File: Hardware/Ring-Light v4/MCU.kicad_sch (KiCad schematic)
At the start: 39 parts, among them U35 CC2640R2FRSMR, U38 W25X40CLUXIG_TR, Y1 32.768kHz, Y2 24MHz

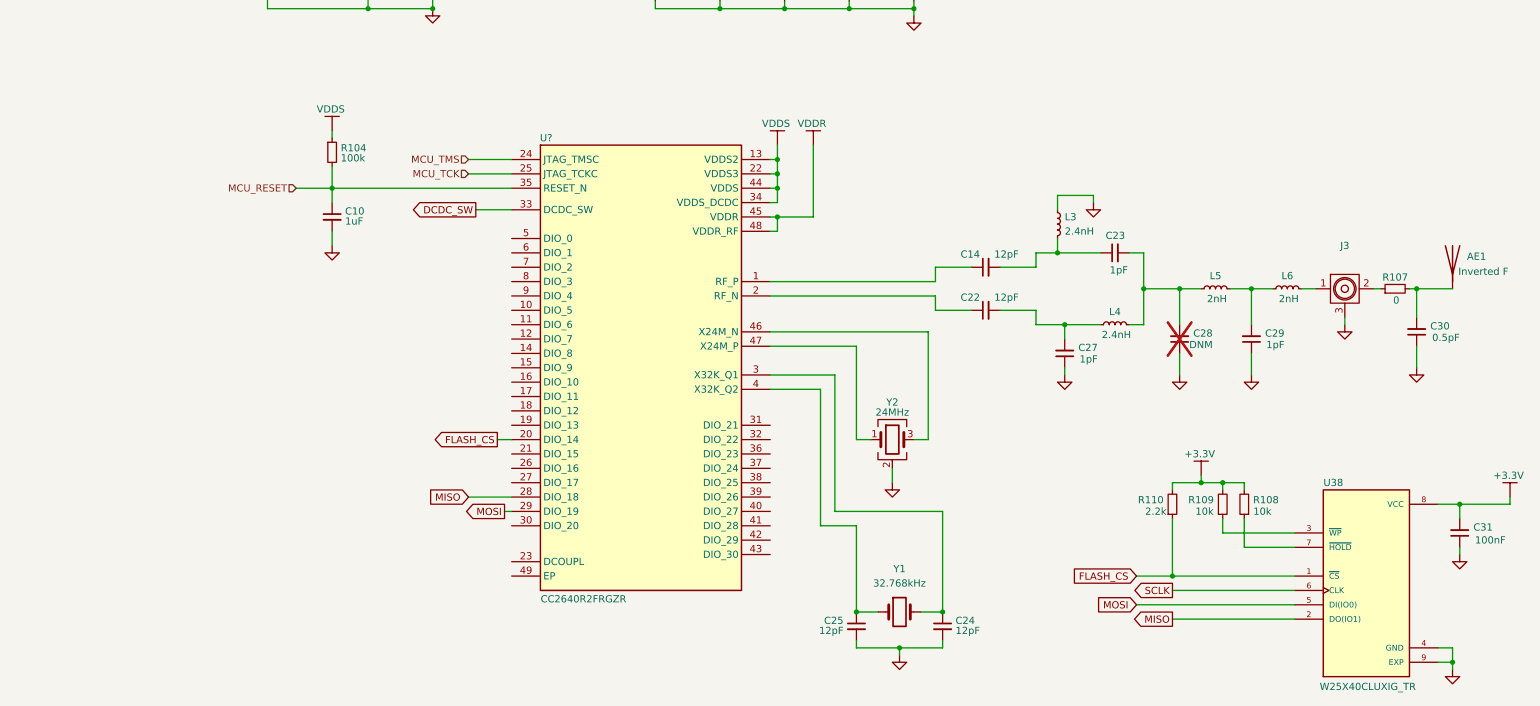
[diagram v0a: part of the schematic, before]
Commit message: m
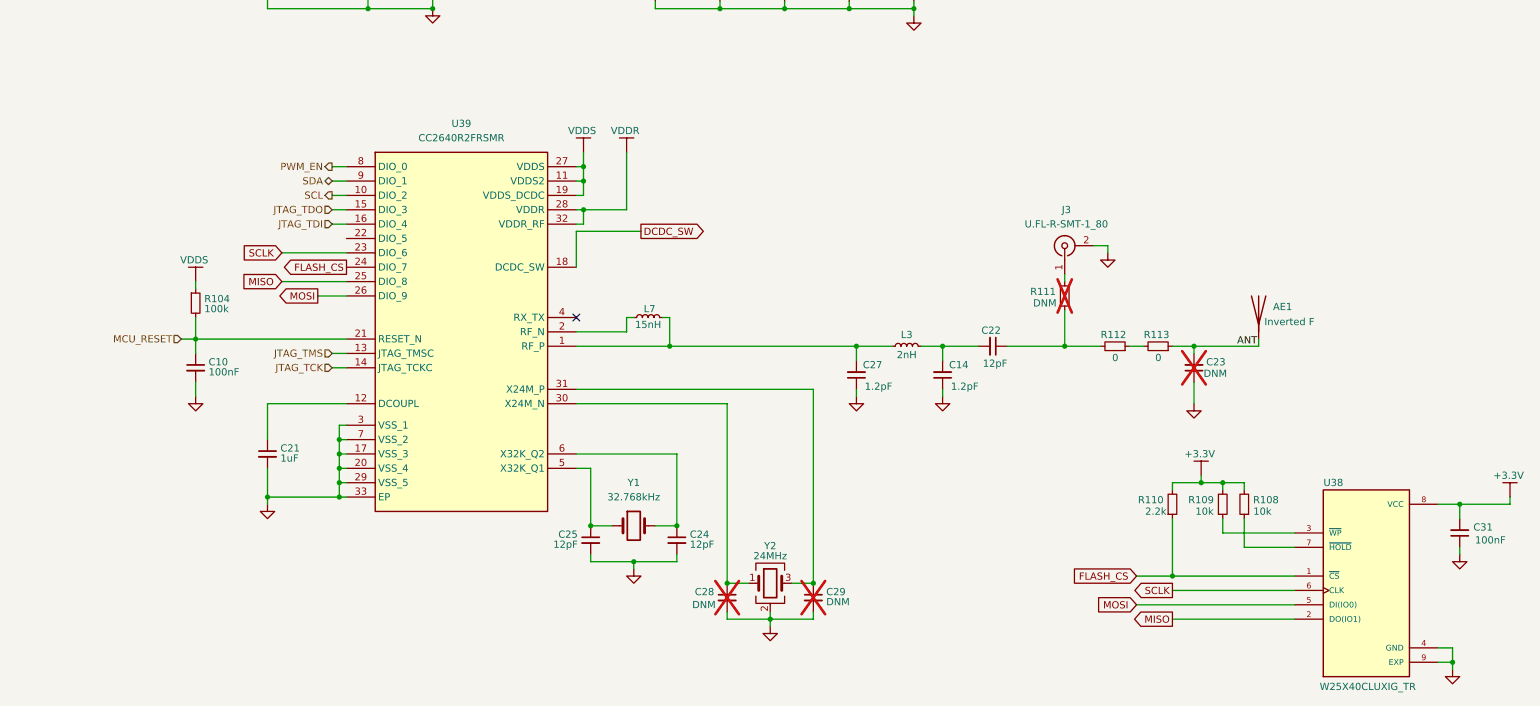
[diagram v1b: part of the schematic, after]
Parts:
- removed C30: 0.5pF, Capacitor_SMD:C_0402_1005Metric, symbol Device:C_Small
- removed J3: ~, symbol Library:M8430-2610RB3
- removed L4: 2.4nH, symbol Device:L_Small
- removed L5, L6: 2nH, symbol Device:L_Small
- removed R107: 0, Resistor_SMD:R_0402_1005Metric, symbol Device:R_Small
- removed U?: CC2640R2FRGZR, QFN50P700X700X100-49N-D, symbol Library:CC2640R2FRGZR
- added C21: 1uF, Capacitor_SMD:C_0402_1005Metric, symbol Device:C_Small
- added J3: U.FL-R-SMT-1_80, Library:UFLRSMT180, symbol Connector:Conn_Coaxial
- added L7: 15nH, symbol Device:L_Small
- added R111: DNM, Resistor_SMD:R_0402_1005Metric, symbol Device:R_Small
- added R112, R113: 0, Resistor_SMD:R_0402_1005Metric, symbol Device:R_Small
- added U39: CC2640R2FRSMR, QFN40P400X400X100-33N-D, symbol Library:CC2640R2FRSMR
- C10: value 1uF -> 100nF
- C14: value 12pF -> 1.2pF
- C23, C29: value 1pF -> DNM; now not fitted
- C27: value 1pF -> 1.2pF
- L3: value 2.4nH -> 2nH
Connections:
- net DCDC_SW: now also U39.18 (DCDC_SW)
- net FLASH_CS: now also U39.24 (DIO_7)
- net GND: now also C14.1, C23.1, C28.2, C29.2, C21.2, J3.2 (Ext), J3.3 (Ext), U39.17 (VSS_3), U39.20 (VSS_4), U39.29 (VSS_5), U39.3 (VSS_1), U39.33 (EP), U39.7 (VSS_2); no longer C28.1, C29.1, L3.1
- net MCU_RESET: now also U39.21 (RESET_N)
- net MISO: now also U39.25 (DIO_8)
- net MOSI: now also U39.26 (DIO_9)
- net SCLK: now also U39.23 (DIO_6)
- net VDDR: now also U39.28 (VDDR), U39.32 (VDDR_RF)
- net VDDS: now also U39.11 (VDDS2), U39.19 (VDDS_DCDC), U39.27 (VDDS)
- net at C27.2: now also L3.1, L7.2, U39.1 (RF_P); no longer C22.2
- net at C14.2, L3.2: now also C22.2; no longer C23.1
- net ANT: now reaches C23.2
- net ANT: now also AE1.1 (A), R113.1; no longer C28.2
- net at C25.1, Y1.1: now also U39.5 (X32K_Q1)
- net at Y2.1: now also C28.1, U39.30 (X24M_N)
- net at Y2.3: now also C29.1, U39.31 (X24M_P)
- net at C22.1: now also R111.1, R112.2
- net at C24.1, Y1.2: now also U39.6 (X32K_Q2)
- new net: R112.1, R113.2
- new net: L7.1, U39.2 (RF_N)
- new net: C21.1, U39.12 (DCOUPL)
- new net: J3.1 (In), R111.2
- new net JTAG_TCK: U39.14 (JTAG_TCKC)
- new net JTAG_TDI: U39.16 (DIO_4)
- new net JTAG_TDO: U39.15 (DIO_3)
- new net JTAG_TMS: U39.13 (JTAG_TMSC)
- new net PWM_EN: U39.8 (DIO_0)
- new net SCL: U39.10 (DIO_2)
- new net SDA: U39.9 (DIO_1)
- no-connect marks 0 -> 1
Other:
- moved on the sheet: AE1, C10, C24, C25, C27, R104, Y1, Y2

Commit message: d
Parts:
- removed C26: 15pF, Capacitor_SMD:C_0402_1005Metric, symbol Device:C_Small
- removed C9: 1uF, Capacitor_SMD:C_0402_1005Metric, symbol Device:C_Small
- removed U35, U39: CC2640R2FRSMR, QFN40P400X400X100-33N-D, symbol Library:CC2640R2FRSMR
- added C20: 1.0uF, Capacitor_SMD:C_0402_1005Metric, symbol Device:C_Small
- added C7, C8: 0.1uF, Capacitor_SMD:C_0402_1005Metric, symbol Device:C_Small
- added D33, D34, D35: TPD1E10B06DPYR, Library:TPD1E10B06DPYR, symbol Diode:ESD5Zxx
- added D36, D37: LTST-C170YKT, Diode_SMD:D_0402_1005Metric, symbol Library:LED
- added J2: 1017457000B11LF, symbol Connector:USB_C_Receptacle
- added J4: Conn_02x05_Counter_Clockwise, symbol Connector_Generic:Conn_02x05_Counter_Clockwise
- added R100, R102, R103, R107, R114: 1k, Resistor_SMD:R_0402_1005Metric, symbol Device:R_Small
- added R105, R106: 100k, Resistor_SMD:R_0402_1005Metric, symbol Device:R_Small
- added U35: CC2640R2FRGZR, QFN50P700X700X100-49N-D, symbol Library:CC2640R2FRGZR
- added U37: CP2102N-A02-GQFN20R, Library:CP2102NA02GQFN20, symbol Library:CP2102N-A02-GQFN20R
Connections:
- net DCDC_SW: now also U35.33 (DCDC_SW)
- net GND: now also C20.2, C7.2, C8.2, D33.2 (A), D34.2 (A), D35.2 (A), J2.13 (SHIELD), J2.A1 (GND), R107.1, R114.1, U35.49 (EP), U37.12 (GND_2), U37.21 (EP_GND), U37.3 (GND_1)
- net JTAG_TCK: now also U35.25 (JTAG_TCKC)
- net JTAG_TMS: now also U35.24 (JTAG_TMSC)
- net MCU_RESET: now also U35.35 (RESET_N)
- net VDDR: now also U35.45 (VDDR), U35.48 (VDDR_RF)
- net VDDS: now also U35.13 (VDDS2), U35.22 (VDDS3), U35.34 (VDDS_DCDC), U35.44 (VDDS)
- net at C27.2, L3.1, L7.2: now also U35.2 (RF_N)
- net at C25.1, Y1.1: now also U35.4 (X32K_Q2)
- net at C28.1, Y2.1: now also U35.47 (X24M_P)
- net at C29.1, Y2.3: now also U35.46 (X24M_N)
- net at L7.1: now also U35.1 (RF_P)
- net at C21.1: now also U35.23 (DCOUPL)
- net at C24.1, Y1.2: now also U35.3 (X32K_Q1)
- new net: C20.1, C8.1, D33.1 (K), J2.A4 (VBUS), J2.B4 (VBUS), U37.7 (VREGIN), U37.8 (VBUS)
- new net: R106.1, U37.17 (RXD)
- new net: R100.2, U37.9 (~{RST})
- new net: J2.B5 (CC2), R114.2
- new net: J2.A5 (CC1), R107.2
- new net: R105.1, U37.18 (TXD)
- new net: D37.1 (K), D37.2 (K), U37.19 (GPIO.3_/_RXT)
- new net: D36.1 (K), D36.2 (K), U37.20 (GPIO.2_/_TXT)
- new net: J2.14 (SHIELD), J2.15 (SHIELD), J2.16 (SHIELD)
- new net D+: D34.1 (K), J2.A6 (D+), J2.B6 (D+), U37.4 (D+)
- new net D-: D35.1 (K), J2.A7 (D-), J2.B7 (D-), U37.5 (D-)
- new net LED_RX: D37.3 (A), D37.4 (A), R103.1
- new net LED_TX: D36.3 (A), D36.4 (A), R102.1
- new net USB_RXD: R106.2
- new net USB_TXD: R105.2
- new net USB_VDD: C7.1, R100.1, R102.2, R103.2, U37.6 (VDD)
- no-connect marks 1 -> 9
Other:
- moved on the sheet: AE1, C10, C11, C12, C13, C14, C15, C16, C17, C18, C19, C21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
